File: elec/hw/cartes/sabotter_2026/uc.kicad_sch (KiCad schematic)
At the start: 37 parts, among them J3 USB4120-03-C, SW1 PTS525 SK15 SMTR2 LFS, U3 ESP32-S3-WROOM-1

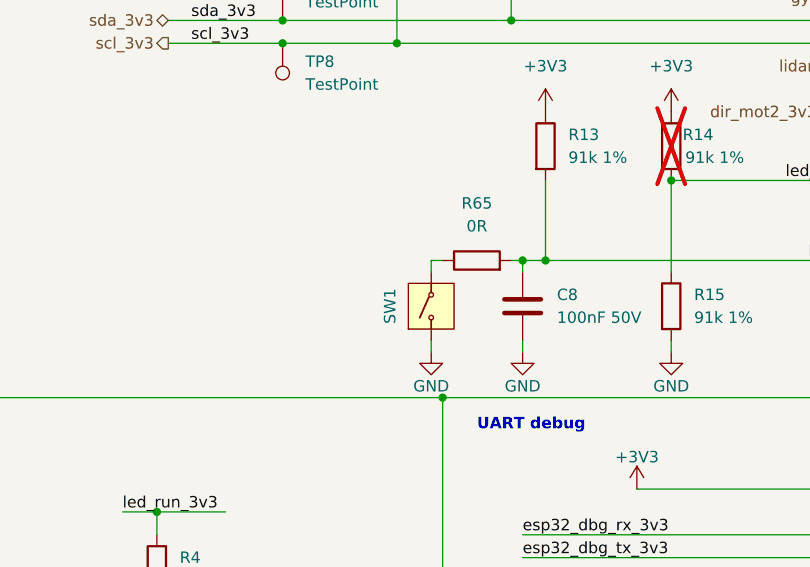
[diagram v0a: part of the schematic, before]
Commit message: sabotter corrections wip
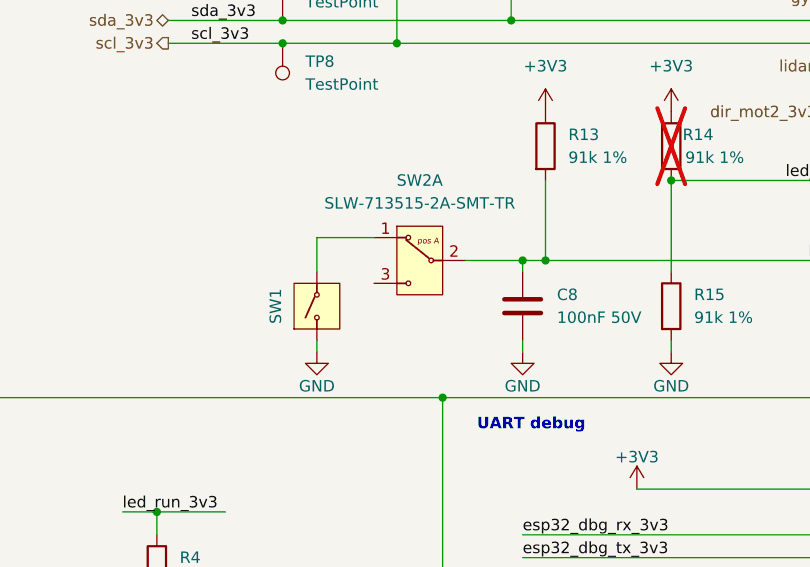
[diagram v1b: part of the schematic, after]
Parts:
- removed R65: 0R, cocotter_resistor:r0603_reflow, symbol cocotter_resistors:R_0R_0603
- added SW2: SLW-713515-2A-SMT-TR, cocotter_others:SLW-713515-2A-SMT-TR, symbol cocotter_connectors:SLW-713515-2A-SMT-TR
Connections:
- net EN_ESP32_3v3: now also SW2.2
- net at SW1.B (2): now also SW2.1
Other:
- moved on the sheet: SW1
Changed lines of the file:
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@@
 	(wire
 		(pts
-			(xy 69.85 152.4) (xy 69.85 153.67)
+			(xy 57.15 152.4) (xy 57.15 153.67)
 		)
 		(stroke
@@
 	(wire
 		(pts
+			(xy 73.66 143.51) (xy 80.01 143.51)
+		)
+		(stroke
+			(width 0)
+			(type default)
+		)
+	)
+	(wire
+		(pts
 			(xy 231.14 149.86) (xy 231.14 151.13)
 		)
@@
 	(wire
 		(pts
-			(xy 69.85 143.51) (xy 69.85 144.78)
+			(xy 57.15 140.97) (xy 57.15 144.78)
 		)
 		(stroke
@@
 	(wire
 		(pts
-			(xy 78.74 143.51) (xy 80.01 143.51)
-		)
-		(stroke
-			(width 0)
-			(type default)
-		)
-	)
-	(wire
-		(pts
 			(xy 104.14 68.58) (xy 104.14 71.12)
 		)
@@
 	(wire
 		(pts
-			(xy 69.85 143.51) (xy 71.12 143.51)
+			(xy 57.15 140.97) (xy 63.5 140.97)
 		)
 		(stroke
@@
 	)
 	(symbol
-		(lib_id "cocotter_resistors:R_0R_0603")
-		(at 74.93 143.51 90)
-		(unit 1)
-		(exclude_from_sim no)
-		(in_bom yes)
-		(on_board yes)
-		(dnp no)
-		(fields_autoplaced yes)
-		(property "Reference" "R65"
-			(at 74.93 137.16 90)
-			(effects
-				(font
-					(size 1.27 1.27)
-				)
-			)
-		)
-		(property "Value" "0R"
-			(at 74.93 139.7 90)
-			(effects
-				(font
-					(size 1.27 1.27)
-				)
-			)
-		)
-		(property "Footprint" "cocotter_resistor:r0603_reflow"
-			(at 74.93 145.288 90)
-			(effects
-				(font
-					(size 1.27 1.27)
-				)
-				(hide yes)
-			)
-		)
-		(property "Datasheet" "~"
-			(at 74.93 143.51 0)
-			(effects
-				(font
-					(size 1.27 1.27)
-				)
-				(hide yes)
-			)
-		)
-		(property "Description" "Resistor"
-			(at 74.93 143.51 0)
-			(effects
-				(font
-					(size 1.27 1.27)
-				)
-				(hide yes)
-			)
-		)
-		(property "Specification" "0R 0603 20mOhms max 100mW"
-			(at 74.93 143.51 0)
-			(effects
-				(font
-					(size 1.27 1.27)
-				)
-				(hide yes)
-			)
-		)
-		(property "mouser" ""
-			(at 74.93 143.51 0)
-			(effects
-				(font
-					(size 1.27 1.27)
-				)
-				(hide yes)
-			)
-		)
-		(property "JLCPCB Part #" "C431718"
-			(at 74.93 143.51 0)
-			(effects
-				(font
-					(size 1.27 1.27)
-				)
-				(hide yes)
-			)
-		)
-		(pin "1"
-		)
-		(pin "2"
-		)
-		(instances
-			(project ""
-				(path "/c1bd5504-d0b2-4cc3-94d1-261f58816249/0627c134-32e1-430c-bbd1-677b8ecf53c1"
-					(reference "R65")
-					(unit 1)
-				)
-			)
-		)
-	)
-	(symbol
 		(lib_id "pmi_2023_specific:+3V3_m")
 		(at 72.39 66.04 0)
@@
 	(symbol
 		(lib_id "cocotter_others:PTS525 SK15 SMTR2 LFS")
-		(at 69.85 148.59 90)
+		(at 57.15 148.59 90)
 		(unit 1)
 		(exclude_from_sim no)
@@
 		(dnp no)
 		(property "Reference" "SW1"
-			(at 65.278 148.59 0)
+			(at 52.578 148.59 0)
 			(effects
 				(font
@@
 		)
 		(property "Value" "PTS525 SK15 SMTR2 LFS"
-			(at 74.93 146.05 0)
+			(at 62.23 146.05 0)
 			(effects
 				(font
@@
 		)
 		(property "Footprint" "cocotter_others:PTS525 SK15 SMTR2 LFS"
-			(at 69.85 148.59 0)
+			(at 57.15 148.59 0)
 			(effects
 				(font
@@
 		)
 		(property "Datasheet" ""
-			(at 74.93 148.59 0)
+			(at 62.23 148.59 0)
 			(effects
 				(font
@@
 		)
 		(property "Description" "20mA max, 15Vdc, 100mohms max, 500k cycle, 260gf"
-			(at 69.85 148.59 0)
+			(at 57.15 148.59 0)
 			(effects
 				(font
@@
 		)
 		(property "JLCPCB Part #" "C2689599"
-			(at 74.93 149.86 0)
+			(at 62.23 149.86 0)
 			(effects
 				(font
@@
 	)
 	(symbol
+		(lib_id "cocotter_connectors:SLW-713515-2A-SMT-TR ")
+		(at 68.58 143.51 0)
+		(unit 1)
+		(exclude_from_sim no)
+		(in_bom yes)
+		(on_board yes)
+		(dnp no)
+		(fields_autoplaced yes)
+		(property "Reference" "SW2"
+			(at 68.58 134.62 0)
+			(effects
+				(font
+					(size 1.27 1.27)
+				)
+			)
+		)
+		(property "Value" "SLW-713515-2A-SMT-TR"
+			(at 68.58 137.16 0)
+			(effects
+				(font
+					(size 1.27 1.27)
+				)
+			)
+		)
+		(property "Footprint" "cocotter_others:SLW-713515-2A-SMT-TR"
+			(at 68.58 143.51 0)
+			(effects
+				(font
+					(size 1.27 1.27)
+				)
+				(hide yes)
+			)
+		)
+		(property "Datasheet" "https://www.sameskydevices.com/product/resource/slw-713515-2a-smt-tr.pdf"
+			(at 68.58 148.59 0)
+			(effects
+				(font
+					(size 1.27 1.27)
+				)
+				(hide yes)
+			)
+		)
+		(property "Description" "50mA max, 12Vdc, 10000 cycles"
+			(at 68.58 143.51 0)
+			(effects
+				(font
+					(size 1.27 1.27)
+				)
+				(hide yes)
+			)
+		)
+		(property "JLCPCB Part #" "C2858291"
+			(at 67.31 148.59 0)
+			(effects
+				(font
+					(size 1.27 1.27)
+				)
+				(hide yes)
+			)
+		)
+		(pin "2"
+		)
+		(pin "1"
+		)
+		(pin "3"
+		)
+		(pin "6"
+		)
+		(pin "4"
+		)
+		(pin "5"
+		)
+		(instances
+			(project ""
+				(path "/c1bd5504-d0b2-4cc3-94d1-261f58816249/0627c134-32e1-430c-bbd1-677b8ecf53c1"
+					(reference "SW2")
+					(unit 1)
+				)
+			)
+		)
+	)
+	(symbol
 		(lib_id "cocotter_resistors:R_0R_0603")
 		(at 120.65 173.99 90)
@@
 	(symbol
 		(lib_id "pmi_2023_specific:GND_m")
-		(at 69.85 153.67 0)
+		(at 57.15 153.67 0)
 		(unit 1)
 		(exclude_from_sim no)
@@
 		(dnp no)
 		(property "Reference" "#PWR14"
-			(at 69.85 160.02 0)
+			(at 57.15 160.02 0)
 			(effects
 				(font
@@
 		)
 		(property "Value" "GND"
-			(at 69.85 157.48 0)
+			(at 57.15 157.48 0)
 			(effects
 				(font
@@
 		)
 		(property "Footprint" ""
-			(at 69.85 153.67 0)
+			(at 57.15 153.67 0)
 			(effects
 				(font
@@
 		)
 		(property "Datasheet" ""
-			(at 69.85 153.67 0)
+			(at 57.15 153.67 0)
 			(effects
 				(font
@@
 		)
 		(property "Description" "Power symbol creates a global label with name \"GND\" , ground"
-			(at 69.85 153.67 0)
+			(at 57.15 153.67 0)
 			(effects
 				(font
